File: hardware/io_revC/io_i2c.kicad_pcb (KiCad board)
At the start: 2 copper layers, 88.9 x 63.5 mm, 15 parts, among them J1 Target Interface, 2716 Pinout, J2 Jumper Block, Q1 2N7000, U1 2716, U2 74HCT74, U3 74HCT125, U4 74HCT138

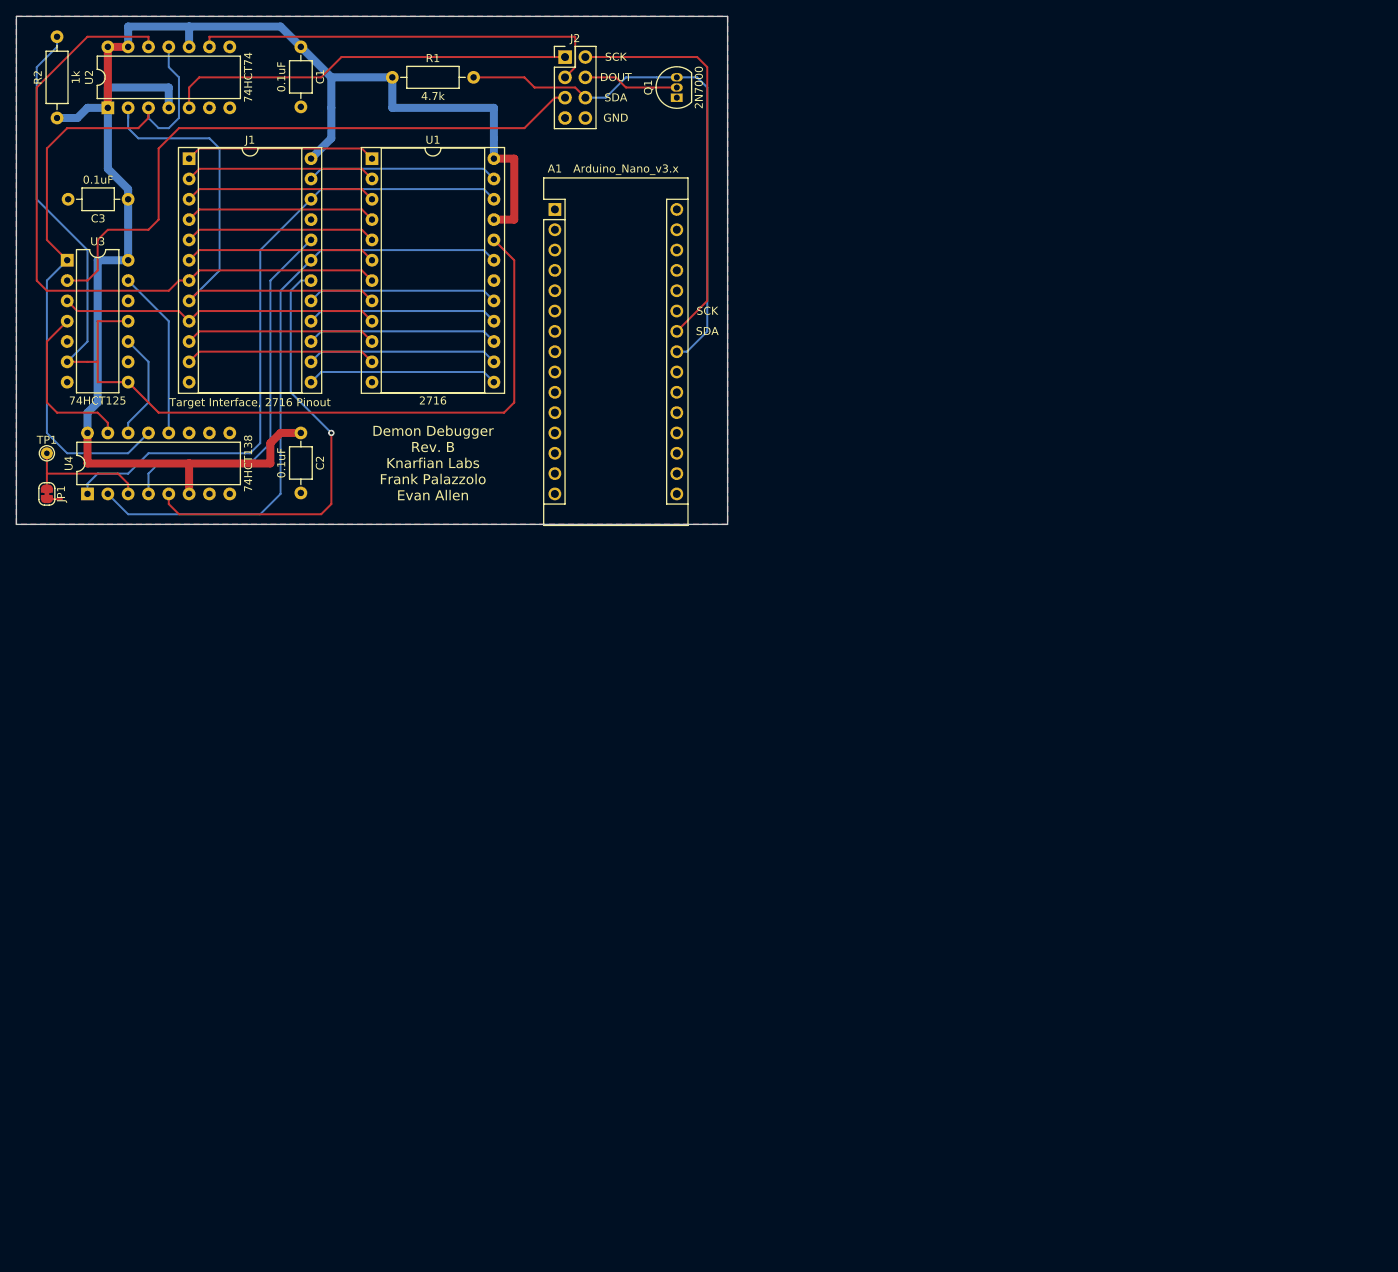
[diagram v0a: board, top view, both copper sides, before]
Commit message: edited for rev C
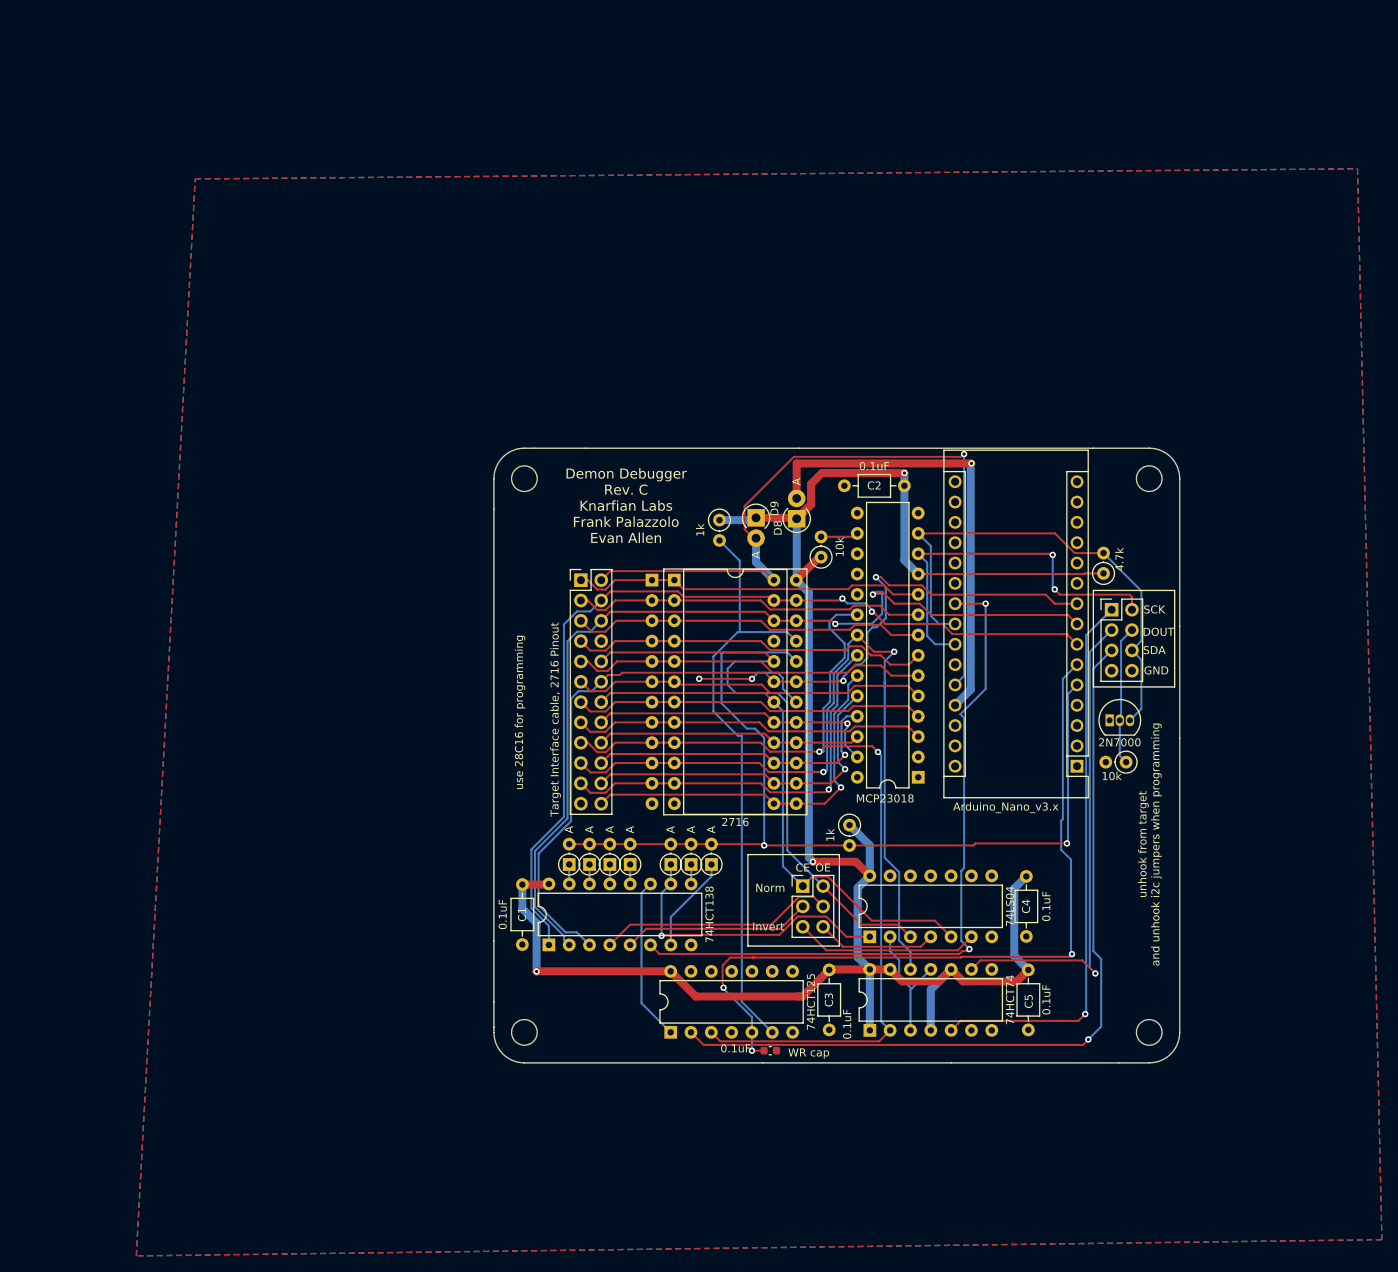
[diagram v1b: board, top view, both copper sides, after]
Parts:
- removed JP1: SolderJumper, Jumper:SolderJumper-2_P1.3mm_Bridged_RoundedPad1.0x1.5mm
- removed TP1: TestPoint, TestPoint:TestPoint_THTPad_D1.5mm_Drill0.7mm
- added C4: 0.1uF, Capacitor_THT:C_Axial_L3.8mm_D2.6mm_P7.50mm_Horizontal, F.Cu at (164.3, 145.6)
- added C5: 0.1uF, Capacitor_THT:C_Axial_L3.8mm_D2.6mm_P7.50mm_Horizontal, F.Cu at (164.6, 157.3)
- added C6: 0.1uF, Capacitor_SMD:C_0603_1608Metric, F.Cu at (132.3, 167.4)
- added D1: 1N4148, Diode_THT:D_DO-35_SOD27_P2.54mm_Vertical_AnodeUp, F.Cu at (107.2, 144.1)
- added D2: 1N4148, Diode_THT:D_DO-35_SOD27_P2.54mm_Vertical_AnodeUp, F.Cu at (109.7, 144.1)
- added D3: 1N4148, Diode_THT:D_DO-35_SOD27_P2.54mm_Vertical_AnodeUp, F.Cu at (112.3, 144.1)
- added D4: 1N4148, Diode_THT:D_DO-35_SOD27_P2.54mm_Vertical_AnodeUp, F.Cu at (114.8, 144.1)
- added D5: 1N4148, Diode_THT:D_DO-35_SOD27_P2.54mm_Vertical_AnodeUp, F.Cu at (119.9, 144.1)
- added D6: 1N4148, Diode_THT:D_DO-35_SOD27_P2.54mm_Vertical_AnodeUp, F.Cu at (122.4, 144.1)
- added D7: 1N4148, Diode_THT:D_DO-35_SOD27_P2.54mm_Vertical_AnodeUp, F.Cu at (125.0, 144.1)
- added D8: 1N4004, Diode_THT:D_DO-41_SOD81_P2.54mm_Vertical_AnodeUp, F.Cu at (130.6, 100.8)
- added D9: 1N4004, Diode_THT:D_DO-41_SOD81_P2.54mm_Vertical_AnodeUp, F.Cu at (135.6, 100.9)
- added J3: Jumper Block, Connector_PinHeader_2.54mm:PinHeader_2x03_P2.54mm_Vertical, F.Cu at (136.4, 146.8)
- added J4: Target Interface cable, 2716 Pinout, Connector_PinHeader_2.54mm:PinHeader_2x12_P2.54mm_Vertical, F.Cu at (108.7, 108.6)
- added R3: 1k, Resistor_THT:R_Axial_DIN0207_L6.3mm_D2.5mm_P2.54mm_Vertical, F.Cu at (126.0, 101.1)
- added R4: 10k, Resistor_THT:R_Axial_DIN0207_L6.3mm_D2.5mm_P2.54mm_Vertical, F.Cu at (176.8, 131.3)
- added R5: 10k, Resistor_THT:R_Axial_DIN0207_L6.3mm_D2.5mm_P2.54mm_Vertical, F.Cu at (138.7, 105.7)
- added REF**: MountingHole_3.2mm_M3, MountingHole:MountingHole_3.2mm_M3, F.Cu at (101.6, 95.9)
- added REF**: MountingHole_3.2mm_M3, MountingHole:MountingHole_3.2mm_M3, F.Cu at (179.7, 95.9)
- added REF**: MountingHole_3.2mm_M3, MountingHole:MountingHole_3.2mm_M3, F.Cu at (101.6, 165.1)
- added REF**: MountingHole_3.2mm_M3, MountingHole:MountingHole_3.2mm_M3, F.Cu at (179.7, 165.1)
- added U5: 74LS04, Package_DIP:DIP-14_W7.62mm, F.Cu at (144.8, 153.2)
- added U6: MCP23018, Package_DIP:DIP-28_W7.62mm, F.Cu at (150.8, 133.2)
- R1, R2: footprint Resistor_THT:R_Axial_DIN0207_L6.3mm_D2.5mm_P10.16mm_Horizontal -> Resistor_THT:R_Axial_DIN0207_L6.3mm_D2.5mm_P2.54mm_Vertical
- moved U2 149.6 mm to (144.8, 164.8)
- moved R2 132.8 mm to (142.2, 139.2), turned to -90 degrees
- moved C3 130.2 mm to (139.7, 157.3), turned to -90 degrees
- moved U3 122.5 mm to (119.9, 165.1), turned to 90 degrees
- moved R1 108.4 mm to (174.0, 107.7), turned to 90 degrees
- moved C1 108.3 mm to (101.3, 146.6)
- moved J2 97.2 mm to (175.0, 112.3)
- moved A1 95.4 mm to (170.7, 131.8), turned to 180 degrees
- moved Q1 94.8 mm to (174.8, 126.1), turned to 0 degrees
- moved U4 80.7 mm to (104.7, 154.2)
- moved J1 78.3 mm to (117.5, 108.6)
- moved C2 75.7 mm to (149.1, 96.8), turned to 180 degrees
- moved U1 64.8 mm to (120.3, 108.6)
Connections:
- A1 pad 1: (no net) -> unconnected-(A1-Pad1)
- A1 pad 10: (no net) -> unconnected-(A1-Pad10)
- A1 pad 11: (no net) -> unconnected-(A1-Pad11)
- A1 pad 12: (no net) -> unconnected-(A1-Pad12)
- A1 pad 13: (no net) -> unconnected-(A1-Pad13)
- A1 pad 14: (no net) -> unconnected-(A1-Pad14)
- A1 pad 15: (no net) -> unconnected-(A1-Pad15)
- A1 pad 16: (no net) -> unconnected-(A1-Pad16)
- A1 pad 17: (no net) -> unconnected-(A1-Pad17)
- A1 pad 18: (no net) -> unconnected-(A1-Pad18)
- A1 pad 19: (no net) -> /no bypass
- A1 pad 2: (no net) -> unconnected-(A1-Pad2)
- A1 pad 20: (no net) -> /bypass
- A1 pad 21: (no net) -> /no RC
- A1 pad 22: (no net) -> /138 enable
- A1 pad 25: (no net) -> unconnected-(A1-Pad25)
- A1 pad 26: (no net) -> +5VD
- A1 pad 27: (no net) -> +5VA
- A1 pad 28: (no net) -> unconnected-(A1-Pad28)
- A1 pad 3: (no net) -> unconnected-(A1-Pad3)
- A1 pad 30: (no net) -> unconnected-(A1-Pad30)
- A1 pad 5: (no net) -> /program OE
- A1 pad 6: (no net) -> /program WR
- A1 pad 7: (no net) -> /A8
- A1 pad 8: (no net) -> /A9
- A1 pad 9: (no net) -> /A10
- J1 pad 18: Net-(J1-Pad18) -> /Target CE
- J1 pad 20: Net-(J1-Pad20) -> /Target OE
- J1 pad 21: (no net) -> unconnected-(J1-Pad21)
- J1 pad 24: +5V -> +5VD
- R2 pad 2: Net-(R2-Pad2) -> /program OE
- U1 pad 20: Net-(R2-Pad2) -> /program OE
- U1 pad 21: +5V -> Net-(U1-Pad21)
- U2 pad 12: /A1 -> /D1
- U2 pad 2: /A0 -> /D0
- U2 pad 6: (no net) -> unconnected-(U2-Pad6)
- U2 pad 8: (no net) -> unconnected-(U2-Pad8)
- U3 pad 1: Net-(U2-Pad11) -> Net-(U3-Pad1)
- U3 pad 10: Net-(U3-Pad10) -> GND
- U3 pad 11: Net-(R2-Pad2) -> unconnected-(U3-Pad11)
- U3 pad 13: Net-(U3-Pad13) -> GND
- U3 pad 4: Net-(U3-Pad4) -> /WR enable
- U3 pad 5: GND -> /program WR
- U3 pad 6: Net-(R2-Pad2) -> Net-(U1-Pad21)
- U3 pad 8: Net-(R2-Pad2) -> unconnected-(U3-Pad8)
- U4 pad 1: /A9 -> /A8
- U4 pad 10: (no net) -> Net-(D5-Pad1)
- U4 pad 11: (no net) -> Net-(U3-Pad1)
- U4 pad 12: Net-(U3-Pad13) -> Net-(D4-Pad1)
- U4 pad 13: Net-(U2-Pad11) -> Net-(D3-Pad1)
- U4 pad 14: Net-(U3-Pad10) -> Net-(D2-Pad1)
- U4 pad 15: Net-(U3-Pad4) -> Net-(D1-Pad1)
- U4 pad 2: /A10 -> /A9
- U4 pad 3: Net-(JP1-Pad1) -> /A10
- U4 pad 4: Net-(J1-Pad20) -> Net-(J3-Pad4)
- U4 pad 5: Net-(J1-Pad18) -> Net-(J3-Pad3)
- U4 pad 6: +5V -> /138 enable
- U4 pad 7: (no net) -> Net-(D7-Pad1)
- U4 pad 9: (no net) -> Net-(D6-Pad1)
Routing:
- net Net-(R2-Pad2): track 136.2 -> 0.00 mm
- net /program OE: track 0.00 -> 119.4 mm, vias 0 -> 2
- net /program WR: track 0.00 -> 95.9 mm, vias 0 -> 3
- net +5VD: track 0.00 -> 92.9 mm, vias 0 -> 1
- net /138 enable: track 0.00 -> 89.9 mm, vias 0 -> 2
- net /A8: track 23.9 -> 111.7 mm, vias 0 -> 2
- net /D0: track 40.2 -> 120.6 mm, vias 0 -> 2
- net /Target OE: track 0.00 -> 77.4 mm
- net Net-(U1-Pad21): track 0.00 -> 74.9 mm
- net /D1: track 23.9 -> 98.7 mm, vias 0 -> 2
- net /Target CE: track 0.00 -> 69.2 mm
- net Net-(U2-Pad11): track 83.6 -> 16.3 mm
- net +5VA: track 0.00 -> 57.3 mm, vias 0 -> 1
- net Net-(J1-Pad18): track 54.5 -> 0.00 mm, vias 1 -> 0
- net +5V: track 200.6 -> 250.8 mm, vias 0 -> 3
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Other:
- board size 88.9 x 63.5 mm -> 85.7 x 76.8 mm
- net class Default removed
- net class Power removed
- board text added: "CE"
- board text added: "Demon Debugger Rev. C Knarfian Labs Frank Palazzolo Evan Allen"
- board text added: "Invert"
- board text added: "Norm"
- board text added: "OE"
- board text added: "WR cap"
- board text added: "unhook from target and unhook i2c jumpers when programming"
- board text added: "use 28C16 for programming"
- board text removed: "Demon Debugger Rev. B Knarfian Labs Frank Palazzolo Evan Allen"
